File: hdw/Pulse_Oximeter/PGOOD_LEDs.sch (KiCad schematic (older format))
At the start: 22 parts, among them U1801 TPS71530, U1802 74LVC1G06, U1803 74LVC1G06, U1804 74LVC1G06, U1805 74LVC1G06, U1806 74LVC1G06

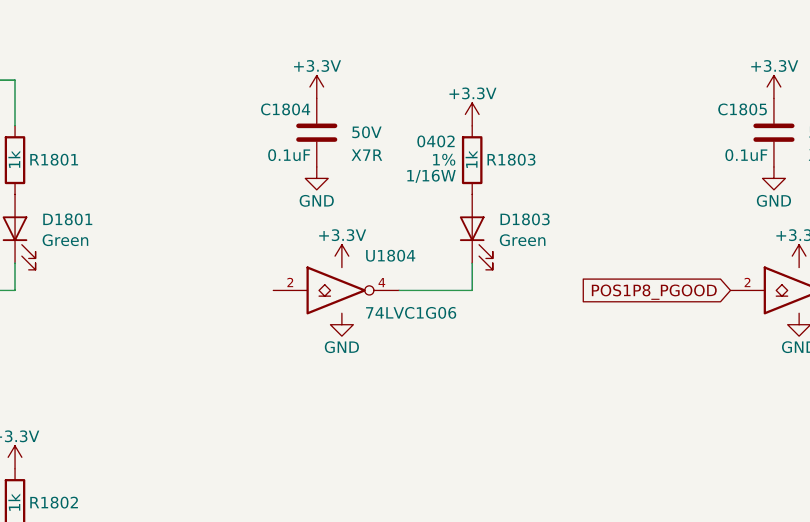
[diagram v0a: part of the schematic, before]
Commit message: few sch additions
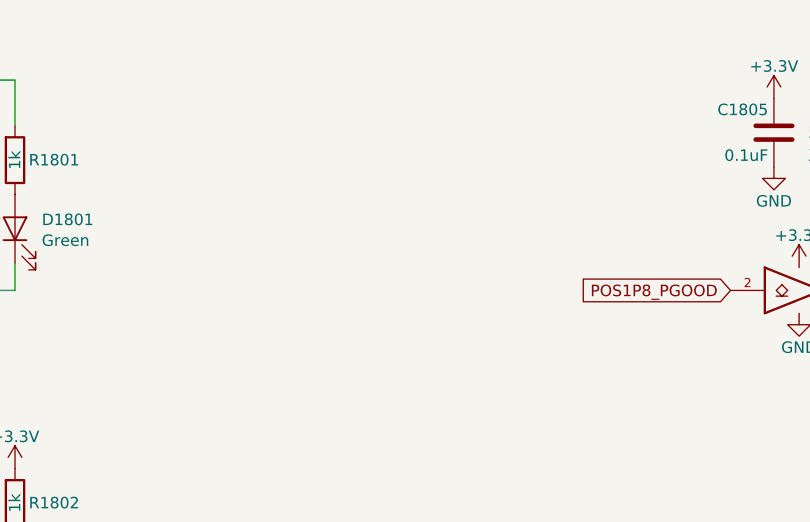
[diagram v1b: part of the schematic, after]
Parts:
- removed C1804: 0.1uF, Capacitors_SMD:C_0402, symbol Custom_Library:C_Custom
- removed D1803: Green, LEDs:LED_0402, symbol Device:LED
- removed R1803: 1k, Resistors_SMD:R_0402, symbol Custom_Library:R_Custom
- removed U1804: 74LVC1G06, TO_SOT_Packages_SMD:SOT-353_SC-70-5, symbol Custom_Library:74LVC1G06_Power
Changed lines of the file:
@@
-$Comp
-L Custom_Library:C_Custom C?
-U 1 1 5CB8C8F5
-P 4870 2180
-AR Path="/5BAAE1F3/5CB8C8F5" Ref="C?"  Part="1"
-AR Path="/5BAAE1CB/5CB8C8F5" Ref="C?"  Part="1"
-AR Path="/5BE48F98/5CB8C8F5" Ref="C?"  Part="1"
-AR Path="/5CAD2D97/5CB8C8F5" Ref="C?"  Part="1"
-AR Path="/5CB7A8BC/5CB8C8F5" Ref="C?"  Part="1"
-AR Path="/5CB7A8C3/5CB8C8F5" Ref="C?"  Part="1"
-AR Path="/5EAE4ADE/5CB8C8F5" Ref="C1804"  Part="1"
-F 0 "C1804" H 4895 2280 50  0000 L CNN
-F 1 "0.1uF" H 4895 2080 50  0000 L CNN
-F 2 "Capacitors_SMD:C_0402" H 4908 2030 50  0001 C CNN
-F 3 "" H 4895 2280 50  0001 C CNN
-F 4 "490-10701-1-ND" H 5295 2680 60  0001 C CNN "Digi-Key PN"
-F 5 "" H 4720 2280 50  0000 R CNN "display_footprint"
-F 6 "50V" H 4720 2180 50  0000 R CNN "Voltage"
-F 7 "X7R" H 4720 2080 50  0000 R CNN "Dielectric"
-	1    4870 2180
-	-1   0    0    -1
-$EndComp
-$Comp
-L Device:LED D?
-U 1 1 5CB8C900
-P 5550 2600
-AR Path="/5BB844FD/5CB8C900" Ref="D?"  Part="1"
-AR Path="/5BF346B3/5CB8C900" Ref="D?"  Part="1"
-AR Path="/5BAAE1F3/5CB8C900" Ref="D?"  Part="1"
-AR Path="/5CAD2D97/5CB8C900" Ref="D?"  Part="1"
-AR Path="/5CB7A8BC/5CB8C900" Ref="D?"  Part="1"
-AR Path="/5CB7A8C3/5CB8C900" Ref="D?"  Part="1"
-AR Path="/5EAE4ADE/5CB8C900" Ref="D1803"  Part="1"
-F 0 "D1803" V 5589 2483 50  0000 R CNN
-F 1 "Green" V 5498 2483 50  0000 R CNN
-F 2 "LEDs:LED_0402" H 5550 2600 50  0001 C CNN
-F 3 "~" H 5550 2600 50  0001 C CNN
-F 4 "1497-1219-1-ND" H 390 -3720 50  0001 C CNN "Digi-Key PN"
-	1    5550 2600
-	0    -1   -1   0
-$EndComp
-Wire Wire Line
-	5230 2870 5550 2870
-Wire Wire Line
-	5550 2870 5550 2750
-$Comp
-L Custom_Library:R_Custom R?
-U 1 1 5CB8C910
-P 5550 2300
-AR Path="/5BAAE1F3/5CB8C910" Ref="R?"  Part="1"
-AR Path="/5BAAE1DC/5CB8C910" Ref="R?"  Part="1"
-AR Path="/5BAAE16C/5CB8C910" Ref="R?"  Part="1"
-AR Path="/5BB844FD/5CB8C910" Ref="R?"  Part="1"
-AR Path="/5BF346B3/5CB8C910" Ref="R?"  Part="1"
-AR Path="/5CAD2D97/5CB8C910" Ref="R?"  Part="1"
-AR Path="/5CB7A8BC/5CB8C910" Ref="R?"  Part="1"
-AR Path="/5CB7A8C3/5CB8C910" Ref="R?"  Part="1"
-AR Path="/5EAE4ADE/5CB8C910" Ref="R1803"  Part="1"
-F 0 "R1803" H 5490 2300 50  0000 R CNN
-F 1 "1k" V 5550 2300 50  0000 C CNN
-F 2 "Resistors_SMD:R_0402" H 5550 2300 50  0001 C CNN
-F 3 "" H 5550 2300 50  0001 C CNN
-F 4 "0402" H 5620 2380 50  0000 L CNN "display_footprint"
-F 5 "1%" H 5620 2300 50  0000 L CNN "Tolerance"
-F 6 "1/16W" H 5620 2230 50  0000 L CNN "Wattage"
-F 7 "541-1.00KLCT-ND" H 5850 2700 60  0001 C CNN "Digi-Key PN"
-	1    5550 2300
-	-1   0    0    -1
-$EndComp
-$Comp
-L power:+3.3V #PWR?
-U 1 1 5CB8C91A
-P 5550 2150
-AR Path="/5CB7A8BC/5CB8C91A" Ref="#PWR?"  Part="1"
-AR Path="/5CB7A8C3/5CB8C91A" Ref="#PWR?"  Part="1"
-AR Path="/5EAE4ADE/5CB8C91A" Ref="#PWR01815"  Part="1"
-F 0 "#PWR01815" H 5550 2000 50  0001 C CNN
-F 1 "+3.3V" H 5550 2290 50  0000 C CNN
-F 2 "" H 5550 2150 50  0001 C CNN
-F 3 "" H 5550 2150 50  0001 C CNN
-	1    5550 2150
-	1    0    0    -1
-$EndComp
-$Comp
-L power:+3.3V #PWR?
-U 1 1 5CB8C924
-P 4980 2770
-AR Path="/5CB7A8BC/5CB8C924" Ref="#PWR?"  Part="1"
-AR Path="/5CB7A8C3/5CB8C924" Ref="#PWR?"  Part="1"
-AR Path="/5EAE4ADE/5CB8C924" Ref="#PWR01813"  Part="1"
-F 0 "#PWR01813" H 4980 2620 50  0001 C CNN
-F 1 "+3.3V" H 4980 2910 50  0000 C CNN
-F 2 "" H 4980 2770 50  0001 C CNN
-F 3 "" H 4980 2770 50  0001 C CNN
-	1    4980 2770
-	1    0    0    -1
-$EndComp
-$Comp
-L power:+3.3V #PWR?
-U 1 1 5CB8C92E
-P 4870 2030
-AR Path="/5CB7A8BC/5CB8C92E" Ref="#PWR?"  Part="1"
-AR Path="/5CB7A8C3/5CB8C92E" Ref="#PWR?"  Part="1"
-AR Path="/5EAE4ADE/5CB8C92E" Ref="#PWR01811"  Part="1"
-F 0 "#PWR01811" H 4870 1880 50  0001 C CNN
-F 1 "+3.3V" H 4870 2170 50  0000 C CNN
-F 2 "" H 4870 2030 50  0001 C CNN
-F 3 "" H 4870 2030 50  0001 C CNN
-	1    4870 2030
-	1    0    0    -1
-$EndComp
-$Comp
-L power:GND #PWR?
-U 1 1 5CB8C938
-P 4980 2970
-AR Path="/5CB7A8BC/5CB8C938" Ref="#PWR?"  Part="1"
-AR Path="/5CB7A8C3/5CB8C938" Ref="#PWR?"  Part="1"
-AR Path="/5EAE4ADE/5CB8C938" Ref="#PWR01814"  Part="1"
-F 0 "#PWR01814" H 4980 2720 50  0001 C CNN
-F 1 "GND" H 4980 2820 50  0000 C CNN
-F 2 "" H 4980 2970 50  0001 C CNN
-F 3 "" H 4980 2970 50  0001 C CNN
-	1    4980 2970
-	1    0    0    -1
-$EndComp
-$Comp
-L power:GND #PWR?
-U 1 1 5CB8C942
-P 4870 2330
-AR Path="/5CB7A8BC/5CB8C942" Ref="#PWR?"  Part="1"
-AR Path="/5CB7A8C3/5CB8C942" Ref="#PWR?"  Part="1"
-AR Path="/5EAE4ADE/5CB8C942" Ref="#PWR01812"  Part="1"
-F 0 "#PWR01812" H 4870 2080 50  0001 C CNN
-F 1 "GND" H 4870 2180 50  0000 C CNN
-F 2 "" H 4870 2330 50  0001 C CNN
-F 3 "" H 4870 2330 50  0001 C CNN
-	1    4870 2330
-	1    0    0    -1
-$EndComp
 $Comp
 L Custom_Library:C_Custom C?
@@
 	1    0    0    -1
 $EndComp
-$Comp
-L Custom_Library:74LVC1G06_Power U1804
-U 1 1 5EBAD160
-P 4980 2870
-F 0 "U1804" H 5080 3020 50  0000 L CNN
-F 1 "74LVC1G06" H 5080 2770 50  0000 L CNN
-F 2 "TO_SOT_Packages_SMD:SOT-353_SC-70-5" H 4980 2920 50  0001 C CNN
-F 3 "http://www.ti.com/lit/ds/symlink/sn74lvc1g06.pdf" H 4980 2870 50  0001 C CNN
-F 4 "296-8484-1-ND" H 4980 2870 50  0001 C CNN "Digi-Key PN"
-	1    4980 2870
-	1    0    0    -1
-$EndComp
